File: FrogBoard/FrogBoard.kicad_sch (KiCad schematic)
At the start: 66 parts, among them J1 Conn_01x10, J10 Conn_01x01, J11 Conn_01x01, J12 Conn_01x01, J13 Conn_01x01, J14 Conn_01x01, J15 Conn_01x01, J16 Conn_01x01, J17 Conn_01x01, J18 Conn_01x01, J19 Conn_01x01, J2 Conn_01x04, J20 Conn_01x01, J21 Conn_01x01, J22 Conn_01x01, J23 Conn_01x01, J24 Conn_01x01, J25 Conn_01x01, J26 USB_B_Micro, J29 Conn_01x01, J3 Conn_01x01, J30 Conn_01x01, J31 Conn_01x01, J32 Conn_01x01, J33 Conn_01x01, J34 Conn_01x01, J35 Conn_01x01, J36 Conn_01x01, J37 Conn_01x01, J4 Stickbox, J5 Conn_01x03_Socket, J6 Conn_01x02, J8 Conn_01x01, J9 Conn_01x01, U1 STM32L432KBUx, U2 USBLC6-2P6, U3 MCP1700T-3302E, U4 BL1555

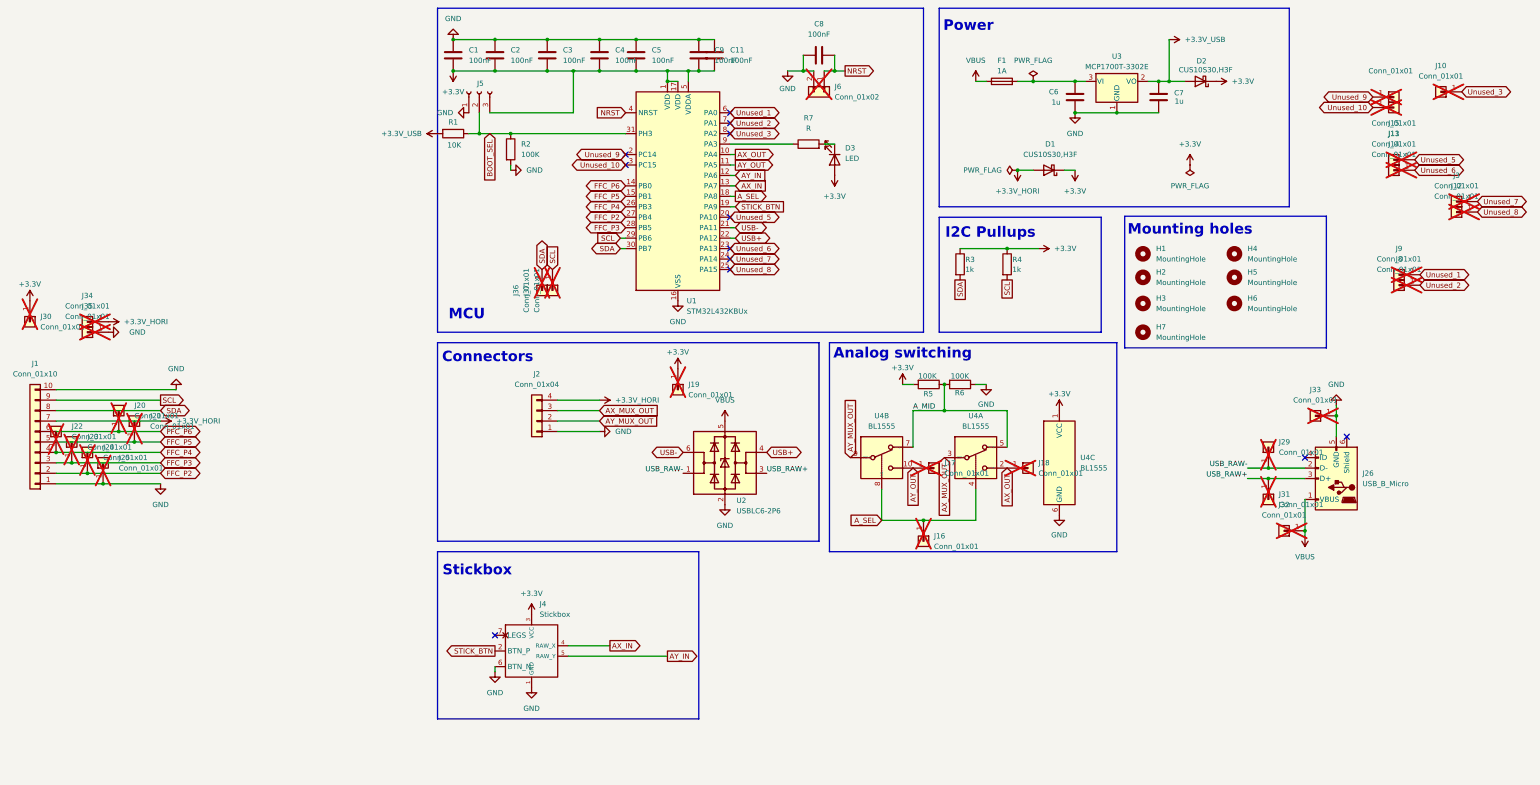
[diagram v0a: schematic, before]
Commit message: Fix silkscreens
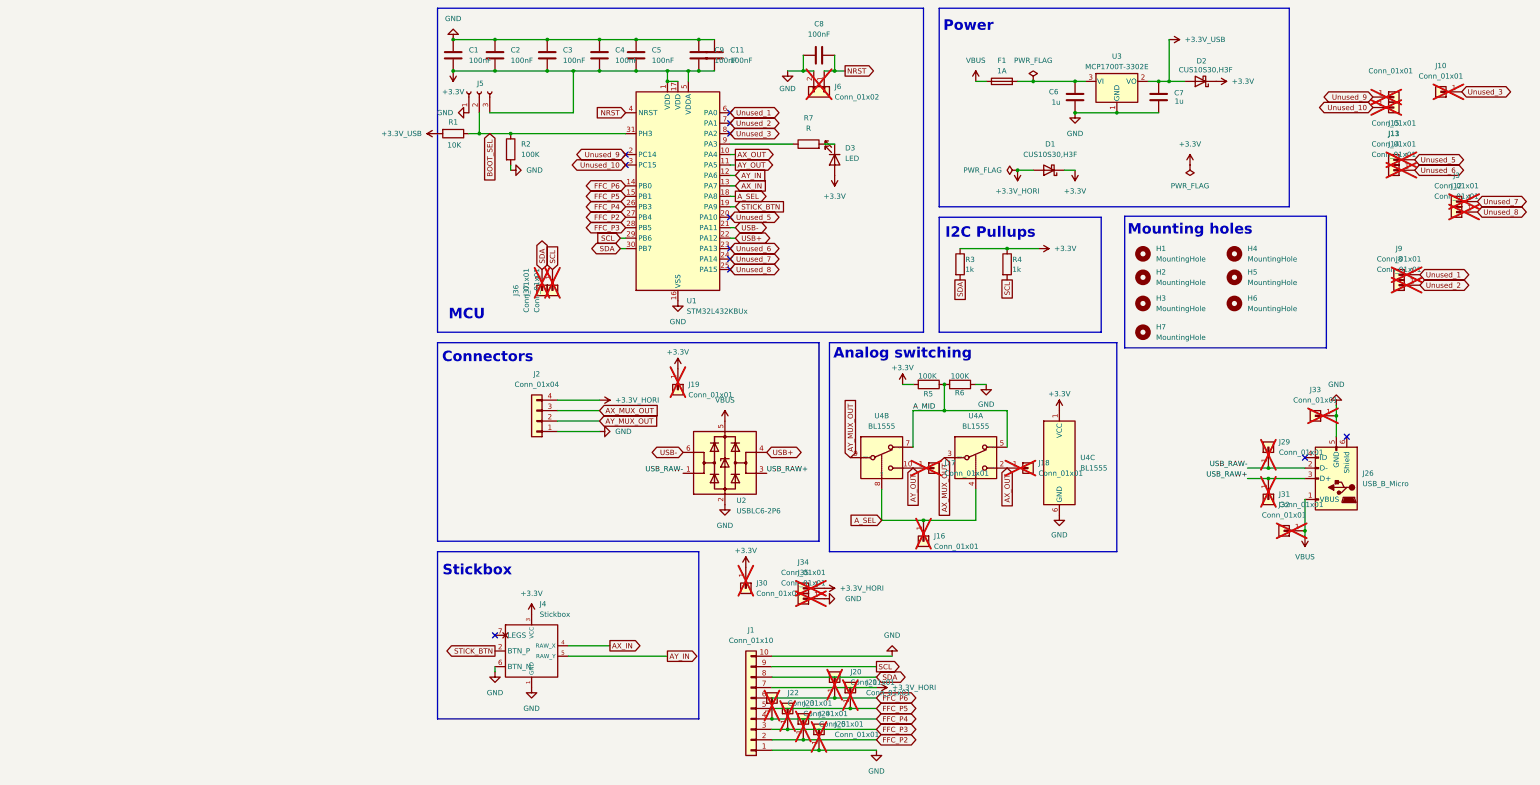
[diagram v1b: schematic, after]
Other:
- moved on the sheet: J1, J20, J21, J22, J23, J24, J25, J30, J34, J35
